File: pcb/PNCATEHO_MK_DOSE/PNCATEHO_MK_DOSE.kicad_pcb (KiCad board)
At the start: 2 copper layers, 97 x 59 mm, 47 parts, among them J1 TestPoint_2Pole, U1 ProMicro_r

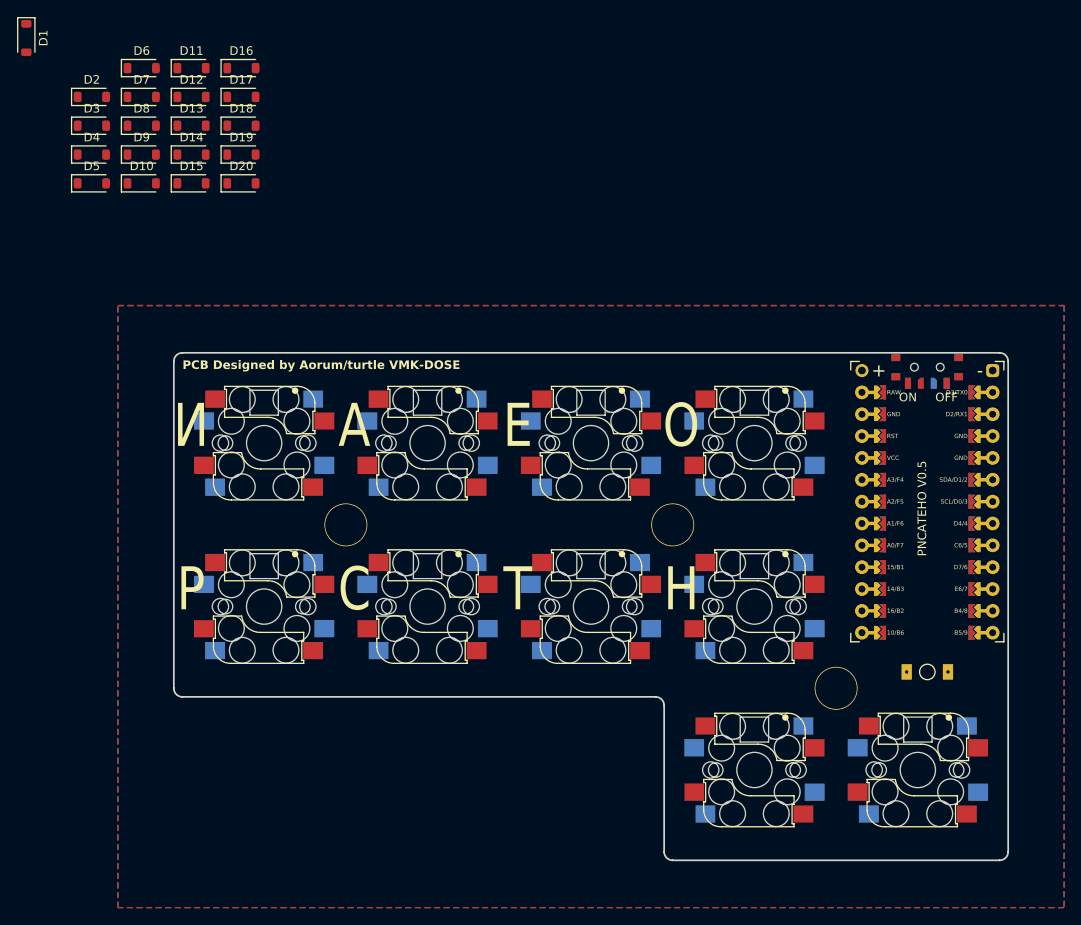
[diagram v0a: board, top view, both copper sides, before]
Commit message: PNCATEHO MK-DOSE routed
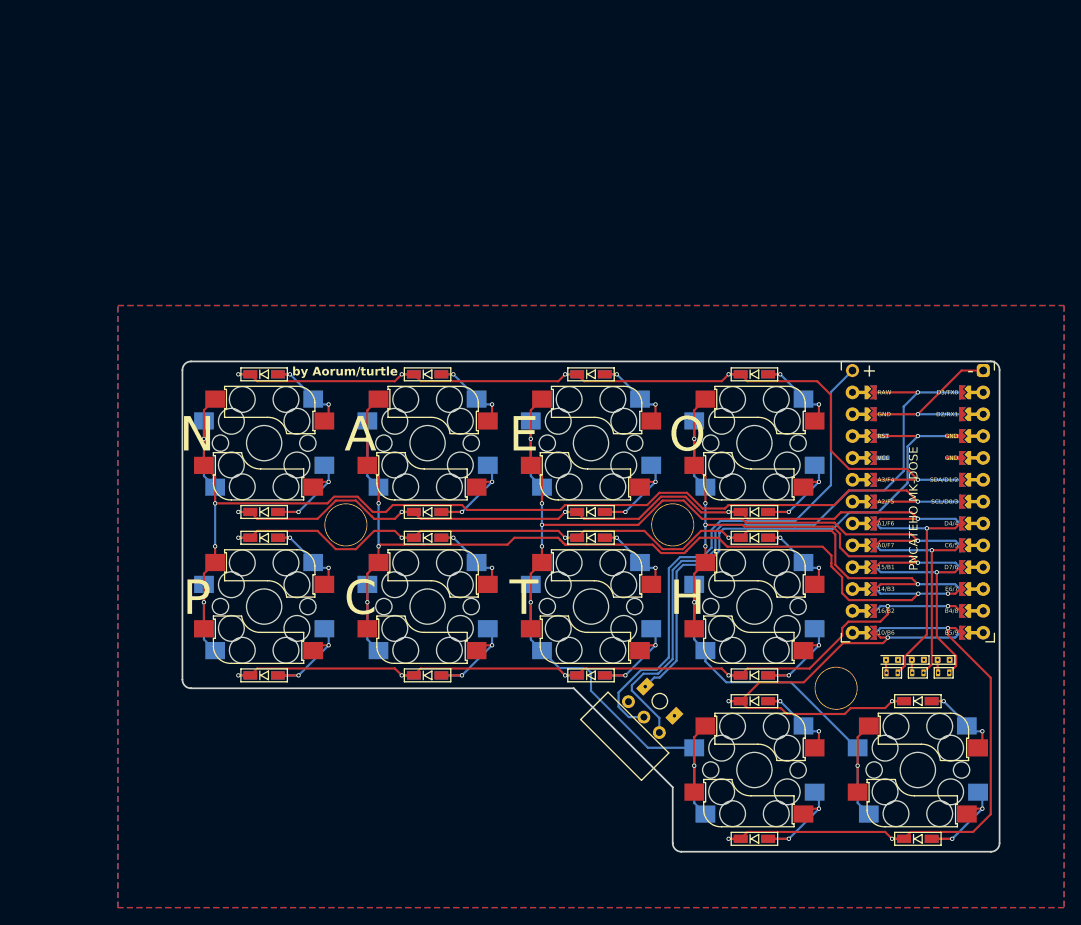
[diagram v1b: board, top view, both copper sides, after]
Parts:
- removed LED1, LED10, LED2, LED3, LED4, LED5, LED6, LED7, LED8, LED9: YS-SK6812MINI-E, PNCATEHO:YS-SK6812MINI-E_duplex
- added D21: LED, PNCATEHO:0603-led_dual, F.Cu at (110.0, 61.2)
- added D22: LED, PNCATEHO:0603-led_dual, F.Cu at (113.0, 61.2)
- added D23: LED, PNCATEHO:0603-led_dual, F.Cu at (116.0, 61.2)
- added R1: R, PNCATEHO:0603-resistor_dual, F.Cu at (110.0, 62.7)
- added R2: R, PNCATEHO:0603-resistor_dual, F.Cu at (113.0, 62.7)
- added R3: R, PNCATEHO:0603-resistor_dual, F.Cu at (116.0, 62.7)
- D1, D10, D11, D12, D13, D14, D15, D16, D17, D18, D19, D2, D20, D3, D4, D5, D6, D7, D8, D9: footprint Diode_SMD:D_SOD-123 -> PNCATEHO:D3_SMD
- PSW1: value SW_SPDT -> ~; footprint PNCATEHO:MSK-12C02_DUAL -> PNCATEHO:bsi10h
- moved D20 109.5 mm to (113.0, 82.0)
- moved D18 102.1 mm to (94.0, 82.0)
- moved D19 101.1 mm to (113.0, 66.0)
- moved D16 92.4 mm to (94.0, 63.0)
- moved D17 92.2 mm to (94.0, 66.0)
- moved D8 84.2 mm to (94.0, 44.0)
- moved D7 78.2 mm to (94.0, 28.0)
- moved D15 77.3 mm to (94.0, 47.0)
- moved D14 76.3 mm to (75.0, 63.0)
- moved D6 73.4 mm to (75.0, 44.0)
- moved D12 72.6 mm to (56.0, 63.0)
- moved D13 66.7 mm to (75.0, 47.0)
- moved D5 62.1 mm to (75.0, 28.0)
- moved D11 61.1 mm to (56.0, 47.0)
- moved D10 58.9 mm to (37.0, 63.0)
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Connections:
- J1 pad 1: Net-(PSW1-B) -> Net-(J1-Pad1)
- PSW1 pad 1: VBAT -> Net-(J1-Pad1)
- PSW1 pad 2: Net-(PSW1-B) -> VBAT
- U1 pad 10: R0 -> C1
- U1 pad 11: R1 -> R3
- U1 pad 12: LED -> R5
- U1 pad 13: R5 -> R4
- U1 pad 14: R4 -> unconnected-(U1-16/B2-Pad14)_1
- U1 pad 15: R3 -> R2
- U1 pad 16: R2 -> C3
- U1 pad 17: C3 -> C2
- U1 pad 18: C2 -> R1
- U1 pad 19: C1 -> C0
- U1 pad 20: C0 -> R0
- U1 pad 21: VCC -> unconnected-(U1-VCC-Pad21)
- U1 pad 7: unconnected-(U1-D4/4-Pad7)_1 -> LED0
- U1 pad 8: unconnected-(U1-C6/5-Pad8)_1 -> LED1
- U1 pad 9: unconnected-(U1-D7/6-Pad9) -> LED2
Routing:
- net C2: track 0.00 -> 142.1 mm, vias 0 -> 7
- net C0: track 0.00 -> 140.9 mm, vias 0 -> 5
- net C1: track 0.00 -> 124.9 mm, vias 0 -> 6
- net C3: track 0.00 -> 122.4 mm, vias 0 -> 7
- net R2: track 0.00 -> 104.6 mm, vias 0 -> 5
- net R0: track 0.00 -> 104.6 mm, vias 0 -> 5
- net R1: track 0.00 -> 100.4 mm, vias 0 -> 5
- net R3: track 0.00 -> 97.1 mm, vias 0 -> 6
- net VBAT: track 0.00 -> 75.7 mm, vias 0 -> 1
- net R5: track 0.00 -> 68.7 mm, vias 0 -> 3
- net reset: track 0.00 -> 63.3 mm, vias 0 -> 1
- net Net-(J1-Pad1): track 0.00 -> 61.4 mm
- net R4: track 0.00 -> 54.5 mm, vias 0 -> 3
- net LED0: track 0.00 -> 28.5 mm, vias 0 -> 1
- net LED1: track 0.00 -> 24.9 mm, vias 0 -> 1
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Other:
- board size 97 x 59 mm -> 95 x 57 mm
- board text added: "A"
- board text added: "C"
- board text added: "E"
- board text added: "H"
- board text added: "N"
- board text added: "O"
- board text added: "P"
- board text added: "PNCATEHO MK-DOSE"
- board text added: "T"
- board text added: "by Aorum/turtle"
- board text removed: "PCB Designed by Aorum/turtle VMK-DOSE"
- board text removed: "PNCATEHO V0.5"
- board text removed: "А"
- board text removed: "Е"
- board text removed: "И"
- board text removed: "Н"
- board text removed: "О"
- board text removed: "Р"
- board text removed: "С"
- board text removed: "Т"
